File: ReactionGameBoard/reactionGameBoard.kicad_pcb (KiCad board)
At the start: 2 copper layers, 53 x 49.7 mm, 15 parts, among them J3 Conn_02x03_Counter_Clockwise, SW1 SW_Push, SW2 SW_DPDT_x2, U1 ATtiny24A-SS, U2 74HC595

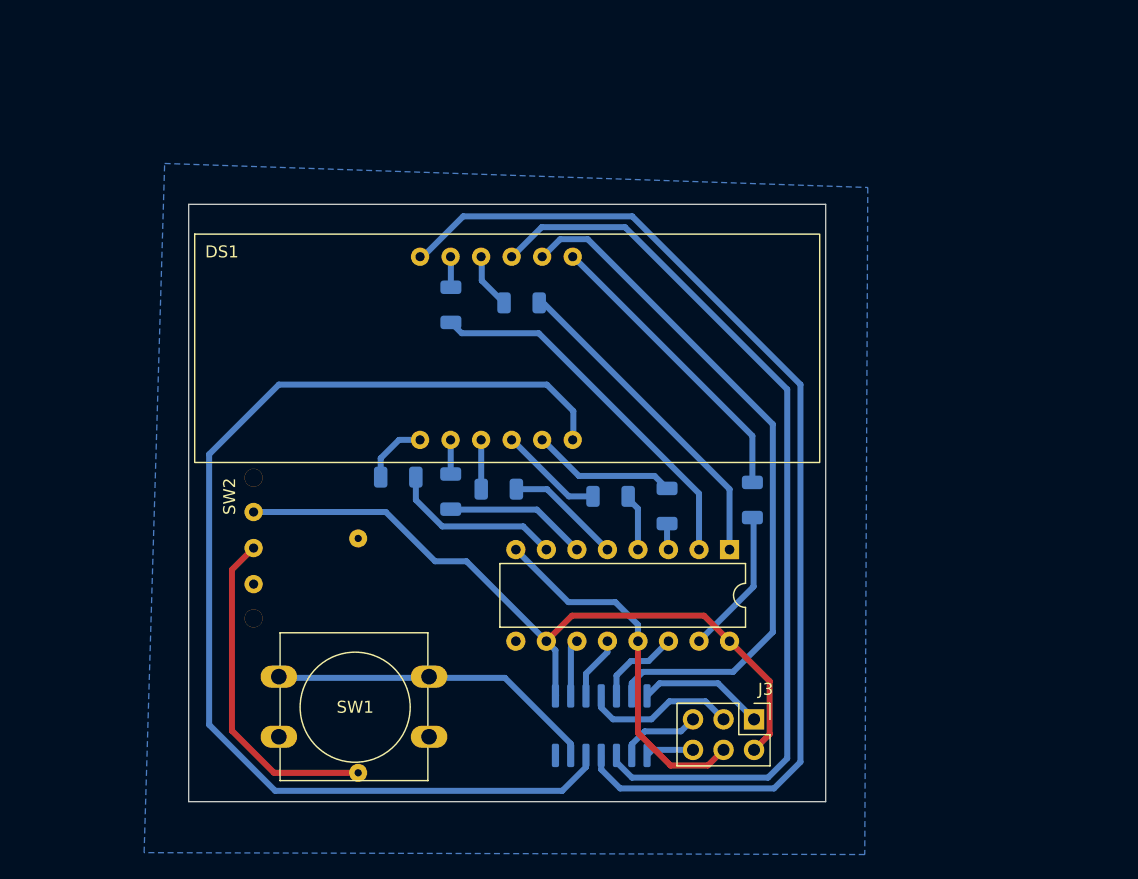
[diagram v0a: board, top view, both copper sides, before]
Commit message: new board design + code
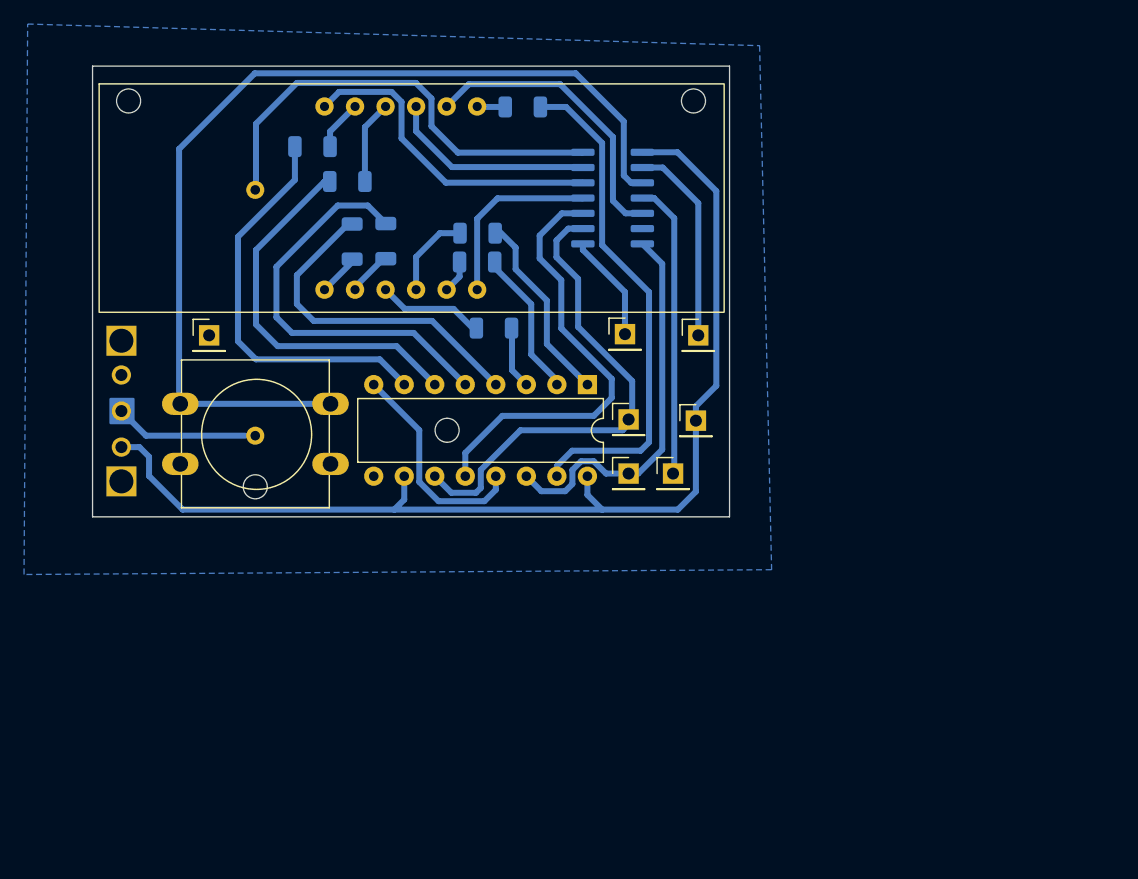
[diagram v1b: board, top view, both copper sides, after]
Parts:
- added H**: hole-2.0mm, CustomParts:hole-2.0mm, F.Cu at (33.0, 25.8)
- added H**: hole-2.0mm, CustomParts:hole-2.0mm, F.Cu at (43.5, 57.9)
- added H**: hole-2.0mm, CustomParts:hole-2.0mm, F.Cu at (80.0, 25.8)
- added H**: hole-2.0mm, CustomParts:hole-2.0mm, F.Cu at (59.5, 53.2)
- added J1: Conn_01x01_Pin, Connector_PinHeader_2.54mm:PinHeader_1x01_P2.54mm_Vertical, F.Cu at (74.6, 56.8)
- added J10: Conn_01x01_Pin, Connector_PinHeader_2.54mm:PinHeader_1x01_P2.54mm_Vertical, F.Cu at (80.2, 52.4)
- added J2: Conn_01x01_Pin, Connector_PinHeader_2.54mm:PinHeader_1x01_P2.54mm_Vertical, F.Cu at (74.3, 45.2)
- added J5: Conn_01x01_Pin, Connector_PinHeader_2.54mm:PinHeader_1x01_P2.54mm_Vertical, F.Cu at (78.3, 56.8)
- added J6: Conn_01x01_Pin, Connector_PinHeader_2.54mm:PinHeader_1x01_P2.54mm_Vertical, F.Cu at (74.6, 52.3)
- added J9: Conn_01x01_Pin, Connector_PinHeader_2.54mm:PinHeader_1x01_P2.54mm_Vertical, F.Cu at (39.7, 45.3)
- J3: value Conn_02x03_Counter_Clockwise -> Conn_01x01_Pin; footprint Connector_PinHeader_2.54mm:PinHeader_2x03_P2.54mm_Vertical -> Connector_PinHeader_2.54mm:PinHeader_1x01_P2.54mm_Vertical
- moved U1 43.9 mm to (73.3, 33.9), turned to 180 degrees
- moved R1 37.9 mm to (65.8, 26.3), turned to 180 degrees
- moved J3 32.3 mm to (80.4, 45.3), turned to 0 degrees
- moved B1 30.2 mm to (43.5, 39.2)
- moved R5 30.2 mm to (51.6, 37.5), turned to -90 degrees
- moved R8 28.4 mm to (48.3, 29.6), turned to 0 degrees
- moved R7 27.2 mm to (51.2, 32.5), turned to 0 degrees
- moved SW1 24.1 mm to (37.3, 51.0)
- moved R6 22.7 mm to (54.4, 37.5), turned to -90 degrees
- moved R4 20.6 mm to (63.4, 44.7), turned to 180 degrees
- moved U2 18.1 mm to (71.2, 49.4)
- moved SW2 15.8 mm to (32.4, 51.6), turned to -90 degrees
- moved DS1 14.8 mm to (55.6, 33.9)
- moved R2 6.86 mm to (62.0, 36.8)
- moved R3 4.18 mm to (62.0, 39.2), turned to 180 degrees
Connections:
- J3 pad 1: MOSI -> serialCS
- R2 pad 2: F -> C
- R3 pad 2: A -> G
- R4 pad 2: G -> Dp
- R5 pad 2: C -> E
- R6 pad 2: Dp -> D
- R7 pad 2: D -> F
- R8 pad 2: E -> A
- SW1 pad 1: PA0 -> PB2
- U1 pad 10: DP2 -> CS2
- U1 pad 11: DP1 -> DP4
- U1 pad 12: DP4 -> DP1
- U1 pad 13: PA0 -> DP2
- U1 pad 2: clock -> serialCS
- U1 pad 3: latch -> PB2
- U1 pad 5: data -> DP3
- U1 pad 6: DP3 -> unconnected-(U1-PA7-Pad6)
- U2 pad 11: clock -> SCK
- U2 pad 12: latch -> CS2
- U2 pad 14: data -> MOSI
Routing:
- net PB2: track 0.00 -> 81.8 mm
- net DP4: track 93.9 -> 15.4 mm
- net DP1: track 89.3 -> 26.9 mm
- net DP2: track 76.1 -> 17.2 mm
- net CS2: track 0.00 -> 36.4 mm
- net SCK: track 6.88 -> 40.6 mm
- net DP3: track 58.0 -> 24.6 mm
- net Net-(U2-QA): track 12.2 -> 42.2 mm
- net +3V0: track 61.7 -> 91.5 mm
- net PA0: track 27.6 -> 0.00 mm
- net GND: track 30.5 -> 56.8 mm
- net Net-(U2-QF): track 9.66 -> 34.3 mm
- net Net-(U2-QE): track 4.57 -> 28.1 mm
- net B: track 25.2 -> 2.35 mm
- net MOSI: track 10.6 -> 32.6 mm
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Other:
- board size 53 x 49.7 mm -> 53 x 37.5 mm

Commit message: cnc pcb version
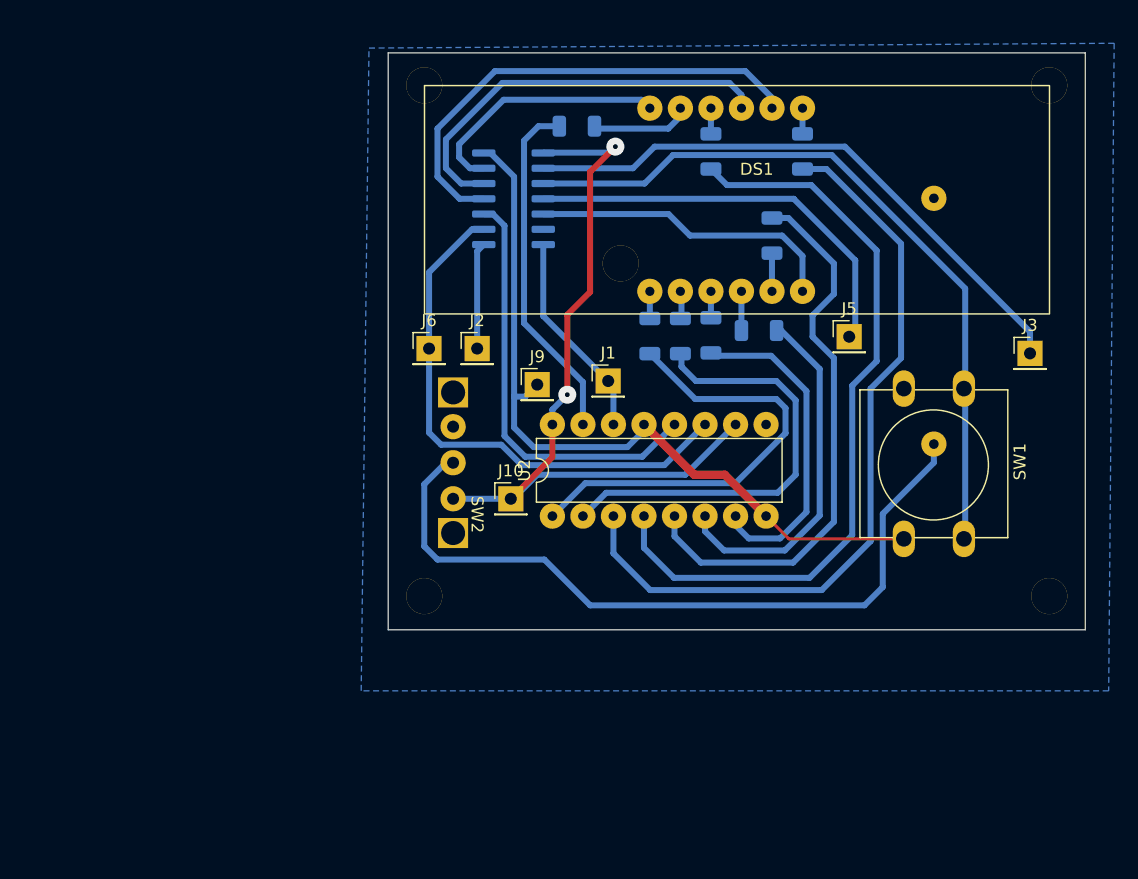
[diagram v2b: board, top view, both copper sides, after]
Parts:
- removed the H** at (33.0, 25.8)
- removed the H** at (43.5, 57.9)
- removed the H** at (80.0, 25.8)
- removed the H** at (59.5, 53.2)
- added H**: hole-3.0mm, CustomParts:hole-3.0mm, F.Cu at (109.6, 67.0)
- added H**: hole-3.0mm, CustomParts:hole-3.0mm, F.Cu at (73.9, 39.3)
- added H**: hole-3.0mm, CustomParts:hole-3.0mm, F.Cu at (109.6, 24.5)
- added H**: hole-3.0mm, CustomParts:hole-3.0mm, F.Cu at (57.6, 24.5)
- added H**: hole-3.0mm, CustomParts:hole-3.0mm, F.Cu at (57.6, 67.0)
- moved SW1 65.2 mm to (102.5, 49.7), turned to -90 degrees
- moved B1 56.5 mm to (100.0, 39.9)
- moved R8 36.7 mm to (81.5, 45.3), turned to 90 degrees
- moved R7 36.4 mm to (85.5, 44.9), turned to 180 degrees
- moved R6 32.1 mm to (86.5, 37.0)
- moved R5 30.8 mm to (81.5, 30.0), turned to 90 degrees
- moved R4 29.6 mm to (89.1, 30.0), turned to 90 degrees
- moved SW2 27.9 mm to (60.0, 55.9)
- moved J3 27.6 mm to (108.0, 46.8)
- moved J9 27.6 mm to (67.0, 49.4)
- moved DS1 27.1 mm to (82.7, 34.0)
- moved J5 18.6 mm to (93.0, 45.4)
- moved R3 18.0 mm to (78.9, 45.4), turned to 90 degrees
- moved J6 17.6 mm to (58.0, 46.4)
- moved J10 16.7 mm to (64.8, 58.9)
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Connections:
- DS1 pad 12: DP1 -> DP2
- DS1 pad 9: DP2 -> DP1
- R1 pad 2: B -> A
- R2 pad 2: C -> E
- R3 pad 2: G -> D
- R4 pad 2: Dp -> B
- R5 pad 2: E -> F
- R6 pad 2: D -> G
- R7 pad 2: F -> C
- R8 pad 2: A -> Dp
- U1 pad 11: DP4 -> DP3
- U1 pad 5: DP3 -> DP4
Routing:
- net Net-(U2-QD): track 5.21 -> 64.0 mm
- net Net-(SW2A-B): track 11.1 -> 62.8 mm
- net Net-(U2-QE): track 28.1 -> 63.6 mm
- net serialCS: track 17.9 -> 49.4 mm
- net +3V0: track 91.5 -> 65.2 mm, vias 0 -> 2
- net Net-(U2-QC): track 12.3 -> 37.1 mm
- net Net-(U2-QB): track 16.4 -> 37.5 mm
- net PB2: track 81.8 -> 61.5 mm
- net DP3: track 24.6 -> 40.2 mm
- net MOSI: track 32.6 -> 17.4 mm
- net Net-(U2-QA): track 42.2 -> 29.1 mm
- net Net-(U2-QF): track 34.3 -> 46.9 mm
- net DP4: track 15.4 -> 26.0 mm
- net reset: track 25.6 -> 34.6 mm
- net GND: track 56.8 -> 64.8 mm
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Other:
- board size 53 x 37.5 mm -> 58 x 48 mm
